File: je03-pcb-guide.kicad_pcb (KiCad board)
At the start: 2 copper layers, 69.8 x 38.1 mm, 26 parts, among them J1 USB4085-GF-A_REVA, SW1 SW_Push, U1 ATmega32U4-AU, Y1 16MHz

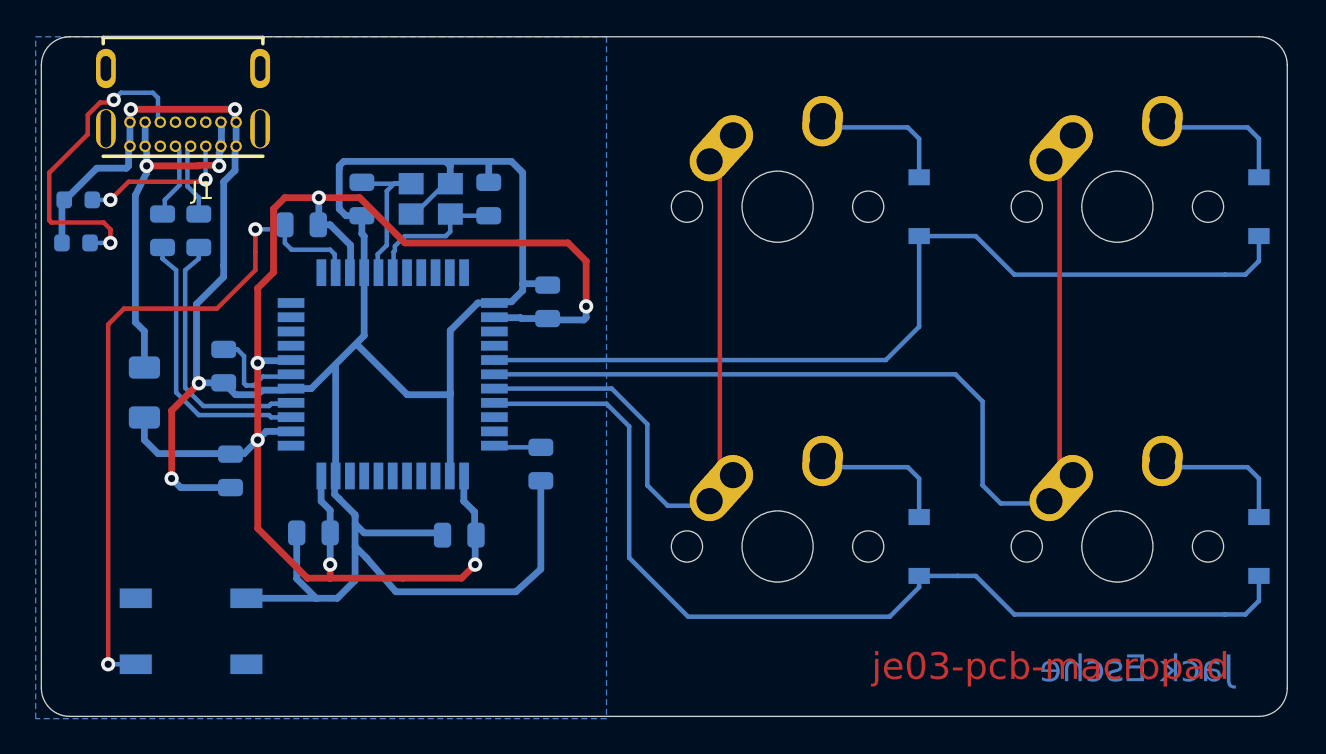
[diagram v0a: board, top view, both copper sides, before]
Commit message: USB-C
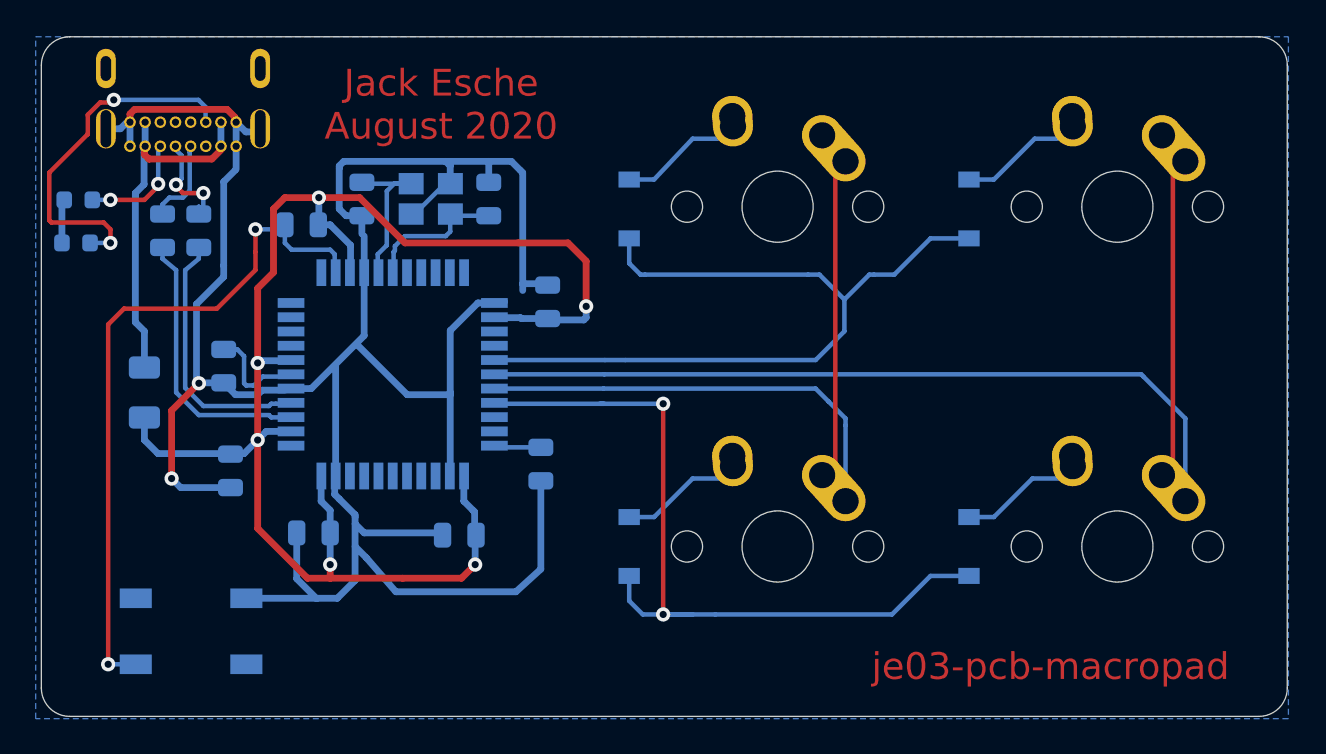
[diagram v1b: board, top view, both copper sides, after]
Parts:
- J1, MX1, MX2, MX3, MX4: moved to B.Cu
- moved D1 16.3 mm to (88.5, 89.0)
- moved D2 16.3 mm to (107.6, 89.0)
- moved D3 16.3 mm to (88.5, 108.0)
- moved D4 16.3 mm to (107.6, 108.0)
- turned J1 to 0 degrees
- turned MX1 to 180 degrees
- turned MX2 to 180 degrees
- turned MX3 to 180 degrees
- turned MX4 to 180 degrees
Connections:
- J1 pad P1: Net-(J1-PadP1) -> GND
- J1 pad P2: Net-(J1-PadP1) -> GND
- J1 pad P3: Net-(J1-PadP1) -> GND
- J1 pad P4: Net-(J1-PadP1) -> GND
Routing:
- net ROW1: track 55.7 -> 44.7 mm, vias 0 -> 2
- net COL0: track 32.9 -> 42.3 mm
- net COL1: track 53.5 -> 61.6 mm
- net ROW0: track 51.1 -> 44.5 mm
- net GND: track 146.3 -> 142.2 mm, vias 4 -> 2
- net Net-(J1-PadA5): track 8.35 -> 6.20 mm
- net Net-(J1-PadB5): track 18.1 -> 20.2 mm
- net D+: track 4.23 -> 6.04 mm, vias 0 -> 2
- net D-: track 4.03 -> 5.06 mm
- net Net-(D2-Pad2): track 6.74 -> 5.90 mm
- net Net-(D1-Pad2): track 6.74 -> 6.19 mm
- net VCC: track 19.7 -> 20.1 mm, vias 2 -> 0
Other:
- board text added: "Jack Esche August 2020"
- board text removed: "Jack Esche"
